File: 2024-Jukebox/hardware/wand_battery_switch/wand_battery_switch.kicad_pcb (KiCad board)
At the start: 2 copper layers, 17.5 x 12 mm, 4 parts, among them J1 Conn_01x02, J2 Conn_01x02, J3 Conn_01x02, SW1 SW_SPDT

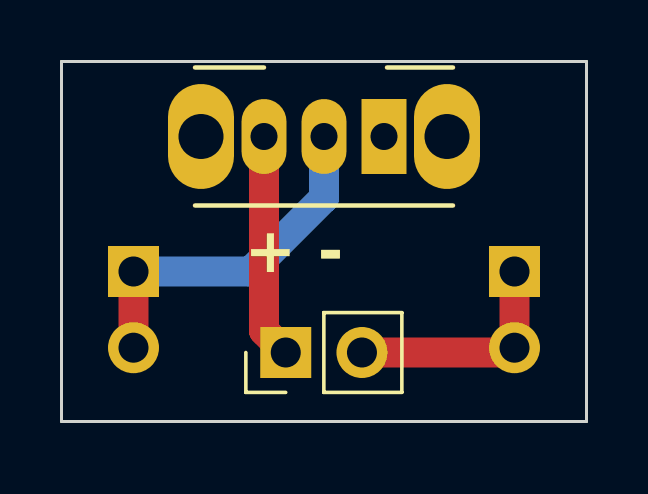
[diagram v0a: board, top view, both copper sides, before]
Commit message: Updated wand PCBs
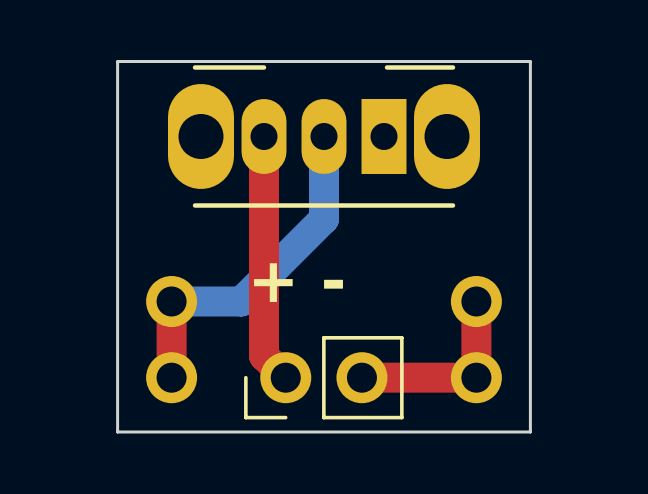
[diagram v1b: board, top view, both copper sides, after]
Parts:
- moved J1 1.62 mm to (3.67, 8.00)
- moved J2 1.62 mm to (13.8, 8.00)
- moved J3 0.84 mm to (7.47, 10.5)
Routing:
- net GND: track 7.69 -> 6.35 mm
- net +BATT: track 7.50 -> 8.34 mm
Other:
- board size 17.5 x 12 mm -> 13.8 x 12.3 mm
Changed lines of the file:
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@@
   (net 4 "Net-(J1-Pin_1)")
   (footprint "Connector_PinHeader_2.54mm:PinHeader_1x02_P2.54mm_Vertical" (layer "F.Cu")
-    (at 7.475 9.7 90)
+    (at 7.475 10.54 90)
     (descr "Through hole straight pin header, 1x02, 2.54mm pitch, single row")
     (tags "Through hole pin header THT 1x02 2.54mm single row")
@@
     (fp_line (start 1.27 3.81) (end -1.27 3.81)
       (stroke (width 0.1) (type solid)) (layer "F.Fab"))
-    (pad "1" thru_hole rect (at 0 0 90) (size 1.7 1.7) (drill 1) (layers "*.Cu" "*.Mask")
+    (pad "1" thru_hole circle (at 0 0 90) (size 1.7 1.7) (drill 1) (layers "*.Cu" "*.Mask")
       (net 2 "+BATT") (pinfunction "Pin_1") (pintype "passive"))
     (pad "2" thru_hole oval (at 0 2.54 90) (size 1.7 1.7) (drill 1) (layers "*.Cu" "*.Mask")
       (net 1 "GND") (pinfunction "Pin_2") (pintype "passive"))
-    (model "${KICAD6_3DMODEL_DIR}/Connector_PinHeader_2.54mm.3dshapes/PinHeader_1x02_P2.54mm_Vertical.wrl"
-      (offset (xyz 0 0 0))
-      (scale (xyz 1 1 1))
-      (rotate (xyz 0 0 0))
-    )
   )
   (footprint "Button_Switch_THT:SW_CuK_OS102011MA1QN1_SPDT_Angled" (layer "F.Cu")
@@
   )
   (footprint "Connector_PinHeader_2.54mm:PinHeader_1x02_P2.54mm_Vertical" (layer "B.Cu")
-    (at 2.4 7 180)
+    (at 3.67 8 180)
     (descr "Through hole straight pin header, 1x02, 2.54mm pitch, single row")
     (tags "Through hole pin header THT 1x02 2.54mm single row")
@@
     (fp_line (start 1.27 1.27) (end 1.27 -3.81)
       (stroke (width 0.1) (type solid)) (layer "B.Fab"))
-    (pad "1" thru_hole rect (at 0 0 180) (size 1.7 1.7) (drill 1) (layers "*.Cu" "*.Mask")
+    (pad "1" thru_hole circle (at 0 0 180) (size 1.7 1.7) (drill 1) (layers "*.Cu" "*.Mask")
       (net 4 "Net-(J1-Pin_1)") (pinfunction "Pin_1") (pintype "passive"))
     (pad "2" thru_hole oval (at 0 -2.54 180) (size 1.7 1.7) (drill 1) (layers "*.Cu" "*.Mask")
@@
   )
   (footprint "Connector_PinHeader_2.54mm:PinHeader_1x02_P2.54mm_Vertical" (layer "B.Cu")
-    (at 15.1 7 180)
+    (at 13.83 8 180)
     (descr "Through hole straight pin header, 1x02, 2.54mm pitch, single row")
     (tags "Through hole pin header THT 1x02 2.54mm single row")
@@
     (fp_line (start 1.27 1.27) (end 1.27 -3.81)
       (stroke (width 0.1) (type solid)) (layer "B.Fab"))
-    (pad "1" thru_hole rect (at 0 0 180) (size 1.7 1.7) (drill 1) (layers "*.Cu" "*.Mask")
+    (pad "1" thru_hole circle (at 0 0 180) (size 1.7 1.7) (drill 1) (layers "*.Cu" "*.Mask")
       (net 1 "GND") (pinfunction "Pin_1") (pintype "passive"))
     (pad "2" thru_hole oval (at 0 -2.54 180) (size 1.7 1.7) (drill 1) (layers "*.Cu" "*.Mask")
@@
     )
   )
-  (gr_rect (start 0 0) (end 17.5 12)
+  (gr_rect (start 1.87 0) (end 15.63 12.35)
     (stroke (width 0.1) (type default)) (fill none) (layer "Edge.Cuts"))
-  (gr_text "+ -" (at 6.1 7.2) (layer "F.SilkS")
+  (gr_text "+ -" (at 6.2 8.2) (layer "F.SilkS")
     (effects (font (size 1.5 1.5) (thickness 0.3) bold) (justify left bottom))
   )
-  (segment (start 15.1 7) (end 15.1 9.54) (width 1) (layer "F.Cu") (net 1))
-  (segment (start 10.015 9.7) (end 14.94 9.7) (width 1) (layer "F.Cu") (net 1))
-  (segment (start 14.94 9.7) (end 15.1 9.54) (width 1) (layer "F.Cu") (net 1))
-  (segment (start 7.475 9.7) (end 6.75 8.975) (width 1) (layer "F.Cu") (net 2))
-  (segment (start 6.75 8.975) (end 6.75 2.5) (width 1) (layer "F.Cu") (net 2))
-  (segment (start 2.4 9.54) (end 2.4 7) (width 1) (layer "F.Cu") (net 4))
-  (segment (start 6.3 7) (end 2.4 7) (width 1) (layer "B.Cu") (net 4))
-  (segment (start 8.75 4.55) (end 6.3 7) (width 1) (layer "B.Cu") (net 4))
-  (segment (start 8.75 2.5) (end 8.75 4.55) (width 1) (layer "B.Cu") (net 4))
+  (segment (start 13.83 8) (end 13.83 10.54) (width 1) (layer "F.Cu") (net 1))
+  (segment (start 10.015 10.54) (end 13.83 10.54) (width 1) (layer "F.Cu") (net 1))
+  (segment (start 6.75 2.5) (end 6.75 9.815) (width 1) (layer "F.Cu") (net 2))
+  (segment (start 6.75 9.815) (end 7.475 10.54) (width 1) (layer "F.Cu") (net 2))
+  (segment (start 3.67 8) (end 3.67 10.54) (width 1) (layer "F.Cu") (net 4))
+  (segment (start 8.75 2.5) (end 8.75 5.25) (width 1) (layer "B.Cu") (net 4))
+  (segment (start 8.75 5.25) (end 6 8) (width 1) (layer "B.Cu") (net 4))
+  (segment (start 6 8) (end 3.67 8) (width 1) (layer "B.Cu") (net 4))
 )
